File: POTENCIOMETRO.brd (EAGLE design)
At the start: 47.8 x 21.5 mm, 13 parts, among them J1 CONECTOR_MACHO, J2 CONECTOR_FEMEA, U1 TL494BD

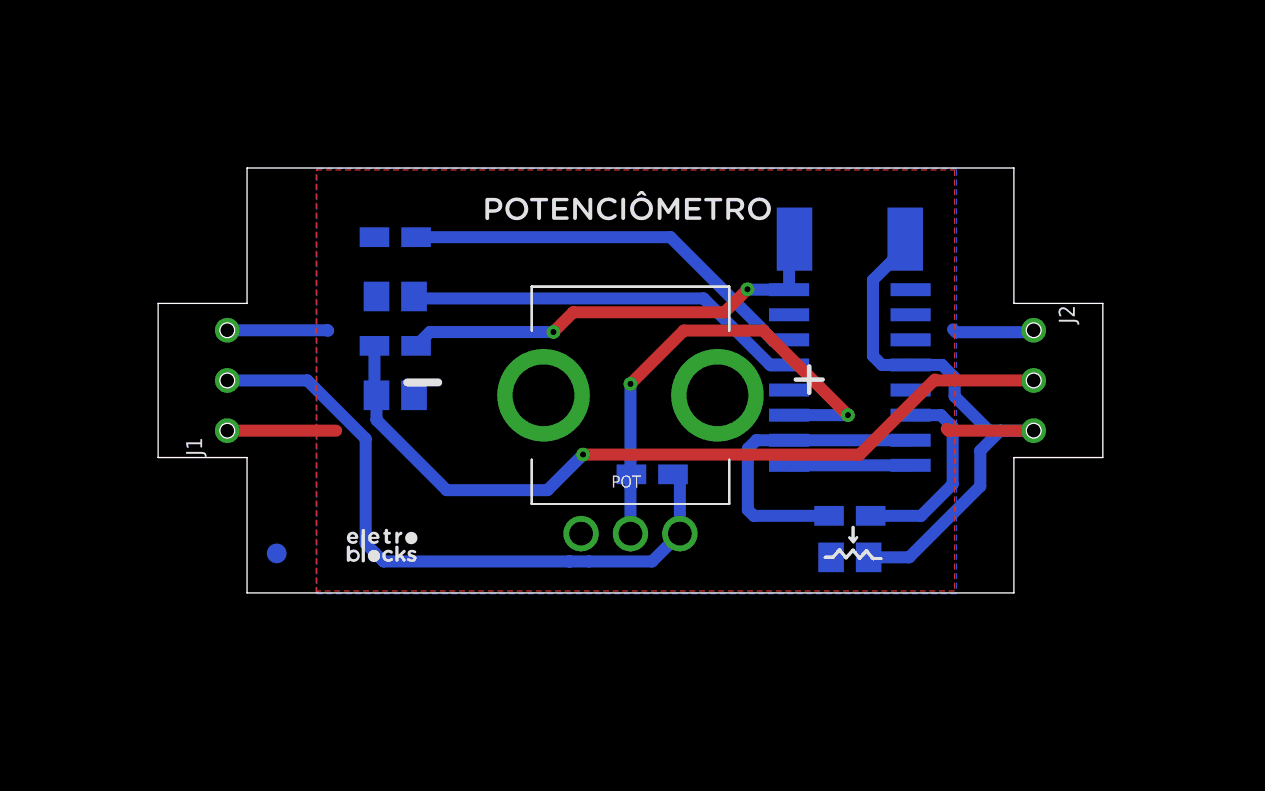
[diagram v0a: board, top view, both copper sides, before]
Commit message: V1.1.1
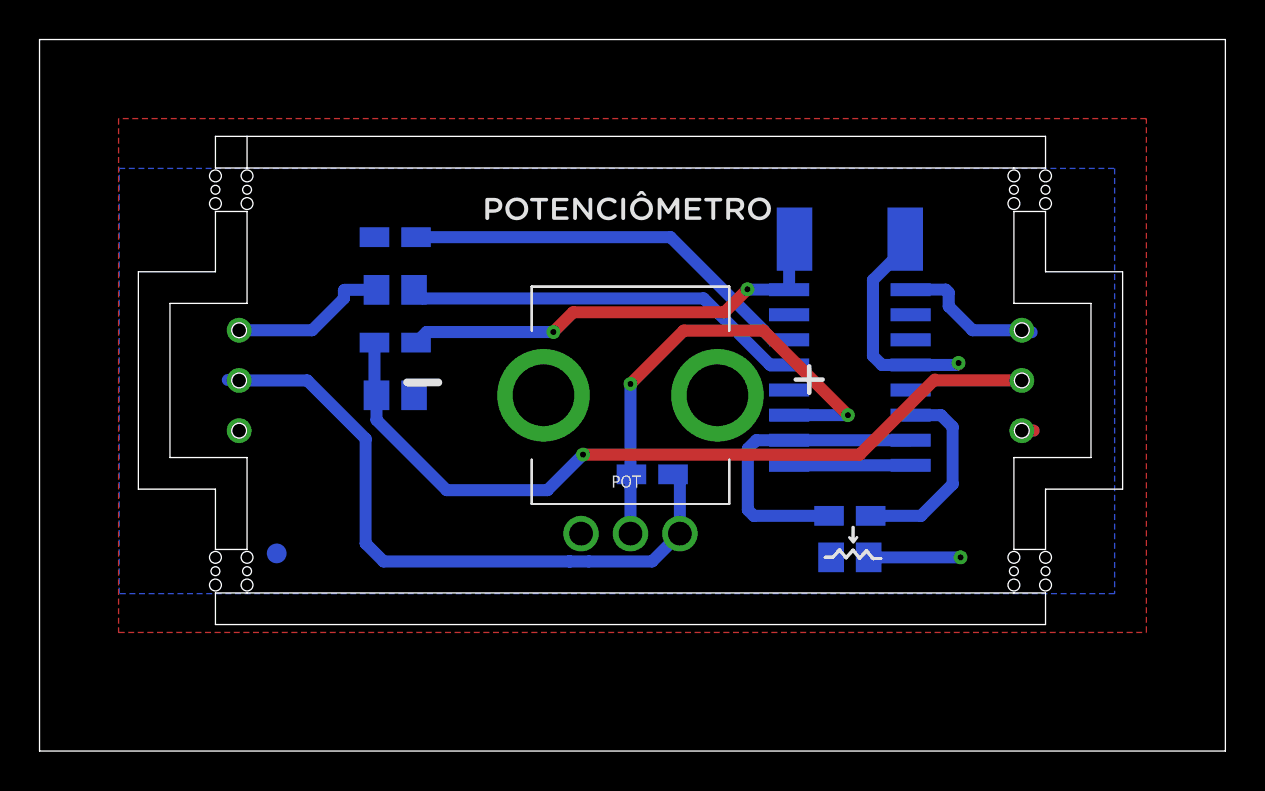
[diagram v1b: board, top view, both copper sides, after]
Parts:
- added U$2, U$3, U$4, U$5: (no value), Eletroblocks Lib:STAMP_DUPLO
- J1: device Eletroblocks Lib:3CONECTOR -> Eletroblocks Lib:MALE
- J2: device Eletroblocks Lib:3CONECTOR -> Eletroblocks Lib:FEMALE
- moved J1 0.60 mm to (-3.90, 10.8)
- moved J2 0.60 mm to (35.7, 10.8)
- moved C2 0.33 mm to (4.00, 15.3)
- moved R5 0.17 mm to (4.00, 12.7)
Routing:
- net VCC: track 38.5 -> 18.4 mm, vias 0 -> 2
- net GND: track 15.4 -> 21.6 mm
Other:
- board size 47.8 x 21.5 mm -> 60 x 36 mm
- board text added: "V1.1.1"
- board text removed: "V1.1.0"
